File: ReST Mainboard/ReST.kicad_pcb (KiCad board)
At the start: 2 copper layers, 100 x 100 mm, 368 parts, among them P20 CONN_02X04, P21 CONN_02X04, P24 CONN_01X03, P26 CONN_01X03, P28 CONN_01X03, P30 CONN_01X03, P32 CONN_01X03, P34 CONN_01X03, P35 SCREW_01X04, P36 SCREW_01X04, P37 SCREW_01X04, P38 SCREW_01X04, P5 USB_OTG, P9 CONN_01X02, U2 USBLC6-2, U4 LM2574N-ADJ

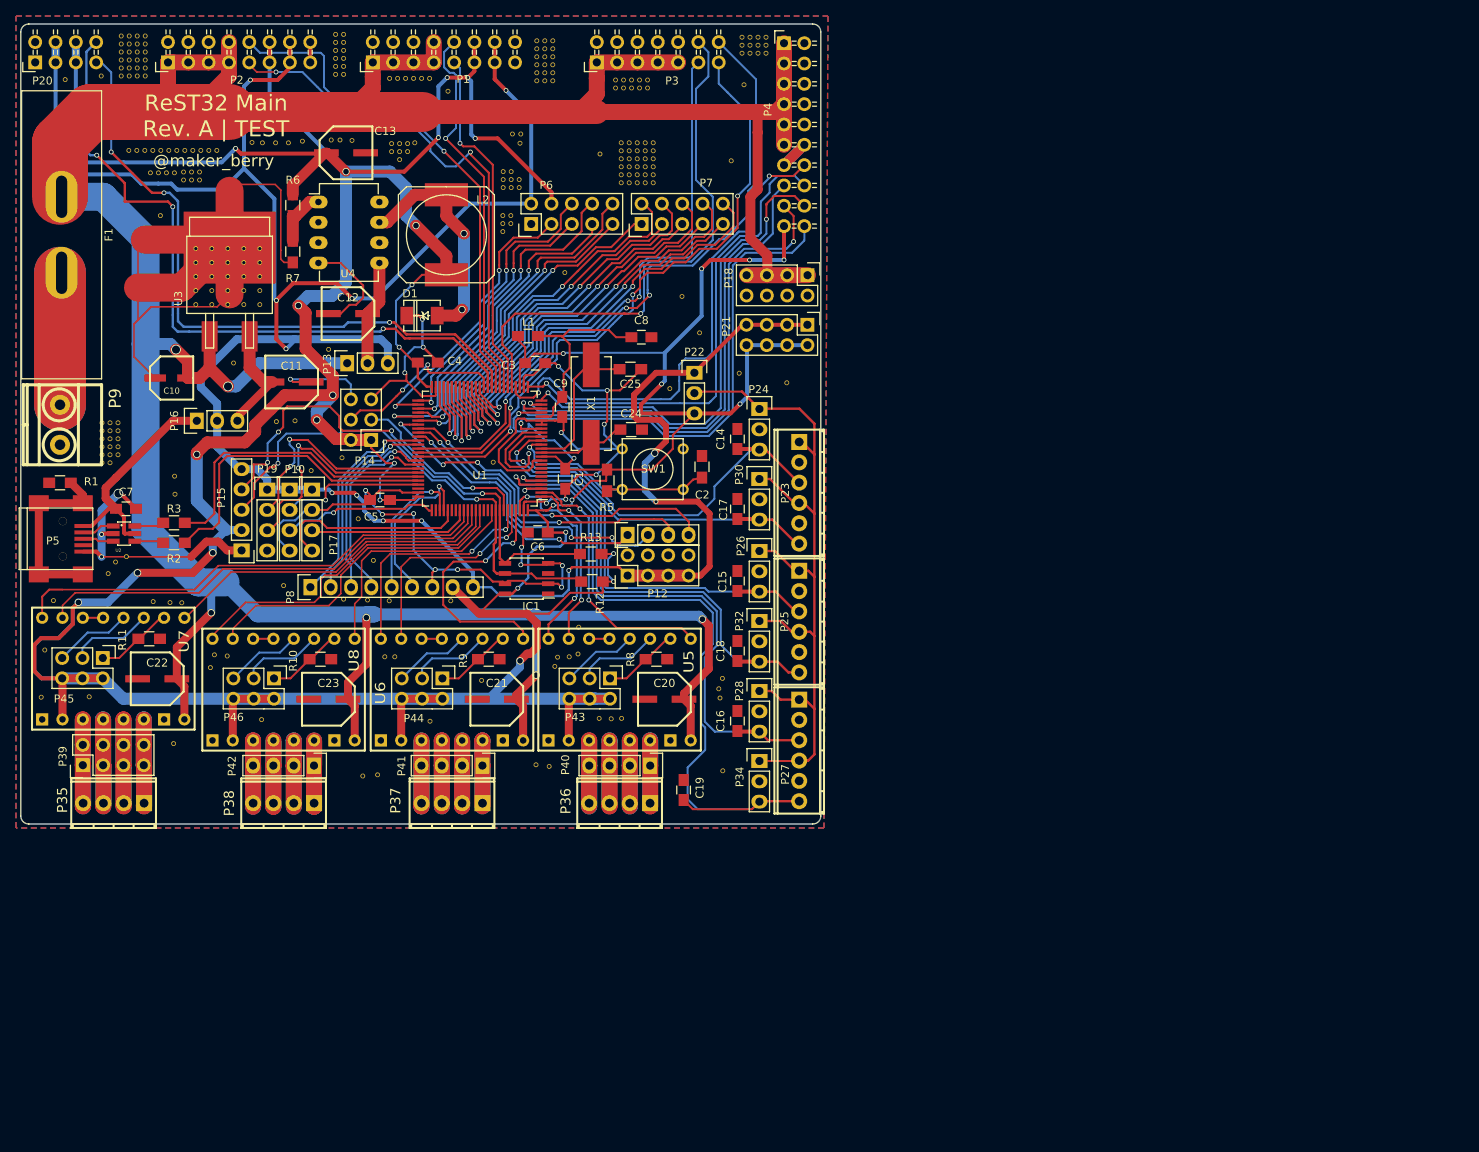
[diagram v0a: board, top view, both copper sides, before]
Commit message: Mainboard structure made and most modules finished
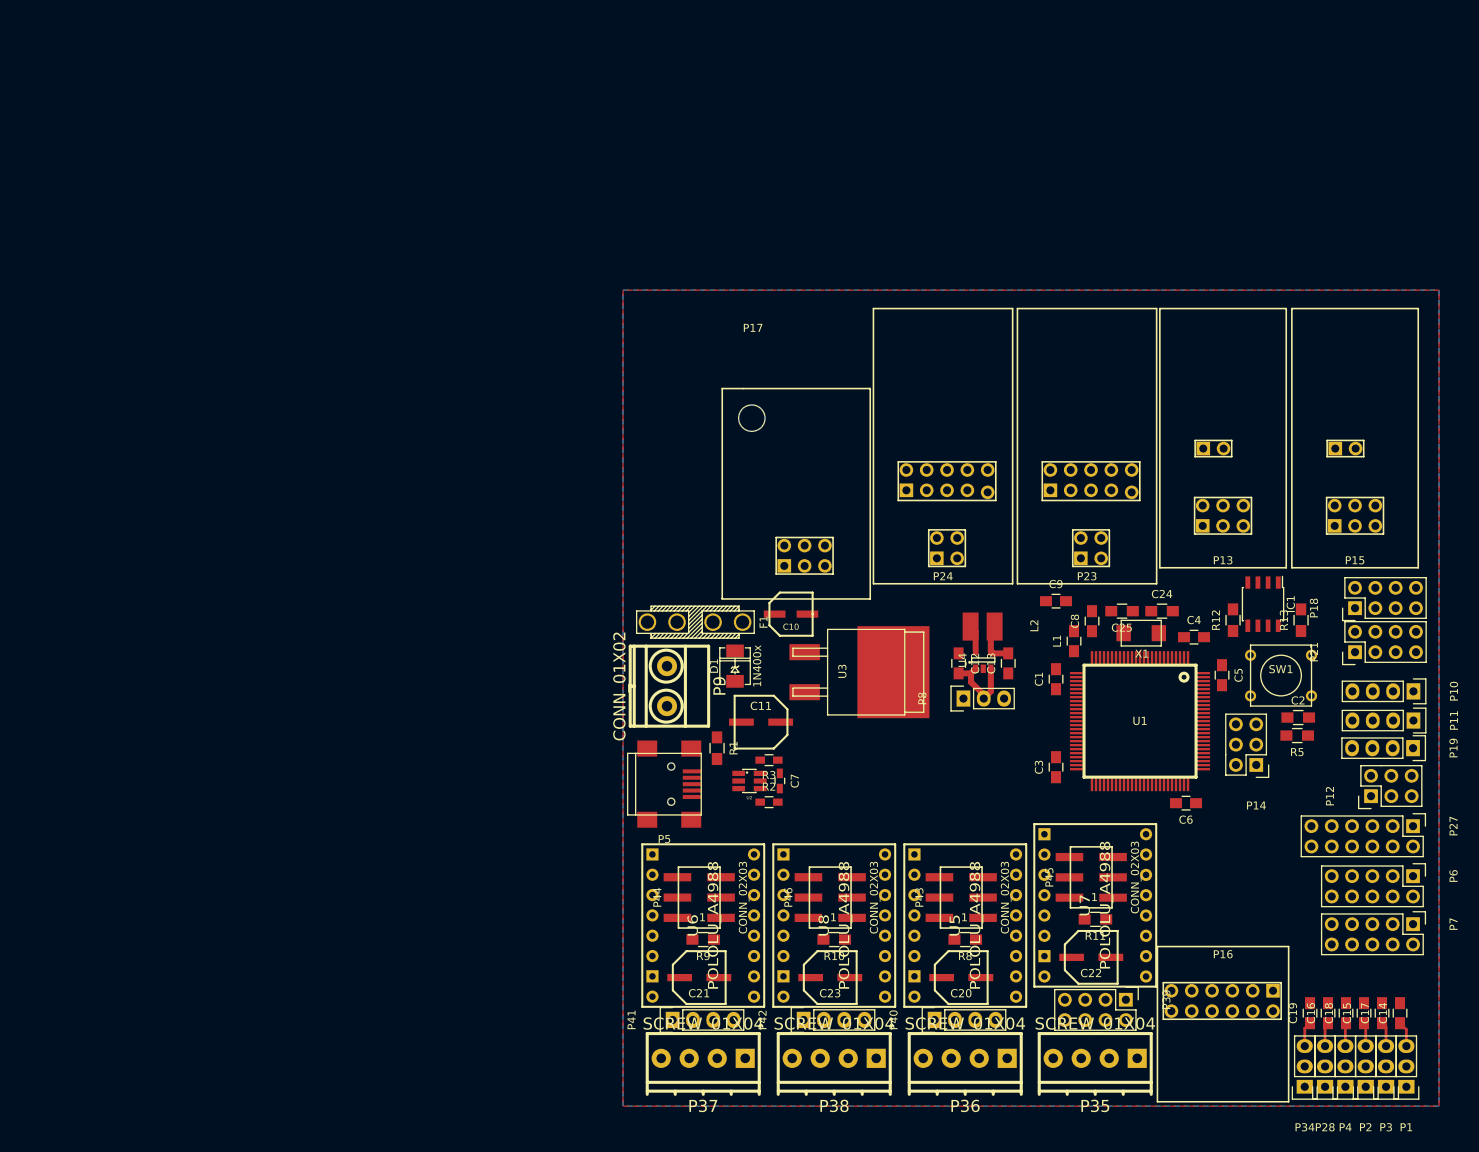
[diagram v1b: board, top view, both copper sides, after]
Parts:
- removed ?: , Pin_Headers:Pin_Header_Straight_1x04
- removed GND (x3), REF**11, REF**111 (x3), REF**11101, REF**1111 (x2), REF**11111 (x2), REF**111111, REF**111112, REF**111113, REF**111114, REF**111115, REF**111116, REF**11112, REF**111121, REF**111122, REF**111123, REF**111124, REF**111125, REF**111126, REF**11113, REF**111131, REF**111132, REF**111133, REF**111134, REF**111135, REF**111136, REF**11114, REF**111141, REF**111142, REF**111143, REF**111144, REF**111145, REF**111146, REF**11115, REF**111151, REF**111152, REF**111153, REF**111154, REF**111155, REF**111156, REF**11116, REF**1112, REF**11121 (x2), REF**11122, REF**11123, REF**11124, REF**11125, REF**11126, REF**1113, REF**1114, REF**1115, REF**1116, REF**112 (x2), REF**1121 (x2), REF**1122, REF**1123, REF**1124, REF**1125, REF**1126, REF**113 (x2), REF**1131 (x2), REF**1132, REF**1133, REF**1134, REF**1135, REF**1136, REF**114 (x2), REF**1141, REF**115 (x2), REF**1151, REF**116 (x2), REF**1161, REF**1171, REF**1181, REF**1191, REF**12, REF**121 (x3), REF**122 (x2), REF**123 (x2), REF**124 (x2), REF**125 (x2), REF**126 (x2), REF**131 (x5), REF**131111 (x6), REF**131112, REF**131113, REF**131114, REF**131115, REF**131121, REF**131122, REF**131123, REF**131124, REF**131125, REF**131131, REF**131132, REF**131133, REF**131134, REF**131135, REF**131141, REF**131142, REF**131143, REF**131144, REF**131145, REF**131151, REF**131152, REF**131153, REF**131154, REF**131155, REF**132 (x2), REF**133 (x2), REF**134 (x2), REF**135 (x2), REF**136, REF**141 (x2), REF**142, REF**143, REF**144, REF**145, REF**146, REF**21, REF**22, REF**31 (x58), REF**311 (x3), REF**3111 (x3), REF**3112 (x2), REF**3113, REF**312 (x3), REF**3121 (x3), REF**3122 (x2), REF**313 (x10), REF**3131 (x2), REF**3132, REF**3141 (x2), REF**3142, REF**3151 (x2), REF**3152, REF**3161, REF**32, REF**321 (x3), REF**322 (x3), REF**323 (x3), REF**331 (x2), REF**332 (x3), REF**333 (x3), REF**341, REF**342, REF**343: VIA-0.6mm, ReST-Library:VIA-0.6mm
- removed GND: , ReST-Library:VIA-0.6mm
- removed P20: CONN_02X04, ReST-Library:Pin_Header_Angled_2x04
- removed P22: , Pin_Headers:Pin_Header_Straight_1x03
- removed P25: , 2:mpt_0,5%2f6-2,54
- removed P26, P30, P32: CONN_01X03, Pin_Headers:Pin_Header_Straight_1x03
- removed R6: 2K7, Resistors_SMD:R_0805_HandSoldering
- removed R7: 1K6, Resistors_SMD:R_0805_HandSoldering
- added P11: CONN_01X04, Pin_Headers:Pin_Header_Straight_1x04, F.Cu at (197.2, 106.8)
- C1, C2, C3, C4, C5, C6, C9: value (none) -> 100nF
- C12: value 22uF -> 10uF; footprint ReST-Library:CP-PANASONIC-SMT_D -> Capacitors_SMD:C_0805_HandSoldering
- C13: value 220uF -> 10uF; footprint ReST-Library:CP-PANASONIC-SMT_D -> Capacitors_SMD:C_0805_HandSoldering
- C14, C15, C16, C17, C18, C19: value (none) -> 10nF
- C24, C25: value (none) -> 30pF
- C7: footprint Capacitors_SMD:C_0805_HandSoldering -> Capacitors_SMD:C_0603_HandSoldering
- C8: value (none) -> 10uF
- D1: value 1N5819 -> 1N400x; footprint ReST-Library:DO-214AC(SMA) -> ReST-Library:DO-214AC.SMA
- F1: footprint ReST-Library:JEF-703C -> ReST-Library:MINI-FUSE
- IC1: value (none) -> AT24C128
- L1: value (none) -> BEAD
- L2: value 330uH -> 2.2uH; footprint Inductors:SELF-WE-PD-XXL -> ReST-Library:CD32
- P1, P2: value (none) -> CONN_01X03; footprint ReST-Library:Pin_Header_Angled_2x08 -> Pin_Headers:Pin_Header_Straight_1x03
- P10, P19, P40, P41, P42: value (none) -> CONN_01X04
- P12: value (none) -> CONN_02X03; footprint Pin_Headers:Pin_Header_Straight_2x04 -> Pin_Headers:Pin_Header_Straight_2x03
- P13: value (none) -> CONN_02X04; footprint Pin_Headers:Pin_Header_Straight_1x03 -> ReST-Library:REST_STEPPER
- P14: value (none) -> CONN_02X03
- P15: value (none) -> CONN_02X04; footprint Pin_Headers:Pin_Header_Straight_1x05 -> ReST-Library:REST_STEPPER
- P16: value (none) -> CONN_02X06; footprint Pin_Headers:Pin_Header_Straight_1x03 -> ReST-Library:REST_ADDITIONAL
- P17: value (none) -> CONN_02X03; footprint Pin_Headers:Pin_Header_Straight_1x04 -> ReST-Library:REST_HEATBED
- P18, P39: value (none) -> CONN_02X04
- P23: value (none) -> CONN_02X07; footprint 2:mpt_0,5%2f6-2,54 -> ReST-Library:REST_HEATER
- P24: value CONN_01X03 -> CONN_02X07; footprint Pin_Headers:Pin_Header_Straight_1x03 -> ReST-Library:REST_HEATER
- P27: value (none) -> CONN_02X06; footprint 2:mpt_0,5%2f6-2,54 -> Pin_Headers:Pin_Header_Straight_2x06
- P3: value (none) -> CONN_01X03; footprint ReST-Library:Pin_Header_Angled_2x07 -> Pin_Headers:Pin_Header_Straight_1x03
- P35, P36, P37, P38: footprint 2:mpt_0,5%2f4-2,54 -> ReST-Library:pt_1,5-4-3,5-h
- P4: value (none) -> CONN_01X03; footprint ReST-Library:Pin_Header_Angled_2x10 -> Pin_Headers:Pin_Header_Straight_1x03
- P43, P44, P45, P46: value (none) -> CONN_02X03; footprint Pin_Headers:Pin_Header_Straight_2x03 -> ReST-Library:bb02-hp06
- P6, P7: value (none) -> CONN_02X05
- P8: value (none) -> CONN_01X03; footprint Pin_Headers:Pin_Header_Straight_1x09 -> Pin_Headers:Pin_Header_Straight_1x03
- P9: footprint 5mm-pitch-terminal:mkds_1,5-2 -> ReST-Library:screw-5-2P
- R10, R11, R8, R9: value (none) -> 100K
- R12, R13: value (none) -> 4K7
- R2, R3: footprint Resistors_SMD:R_0805_HandSoldering -> Resistors_SMD:R_0603_HandSoldering
- R5: value (none) -> 10K
- SW1: value (none) -> SW-SPST-NO
- U1: value (none) -> STM32F103VE; footprint Housings_QFP:TQFP-100_14x14mm_Pitch0.5mm -> ReST-Library:LQFP100-14x14
- U3: value (none) -> L7805ACD2T-TR
- U4: value LM2574N-ADJ -> LM3671MFX-3.3; footprint Housings_DIP:DIP-8_W7.62mm_LongPads -> TO_SOT_Packages_SMD:SOT-23-5
- U5, U6, U7, U8: value (none) -> POLOLU_A4988
- X1: value (none) -> Crystal_Small; footprint Crystals:Crystal_HC49-SD_SMD -> ReST-Library:2P-5032
- moved P2 197.0 mm to (191.3, 152.5), turned to 180 degrees
- moved P1 181.9 mm to (196.4, 152.5), turned to 180 degrees
- moved P3 161.6 mm to (193.8, 152.5), turned to 180 degrees
- moved P16 148.8 mm to (173.4, 144.7), turned to 180 degrees
- moved P4 148.1 mm to (188.7, 152.5), turned to 180 degrees
- moved P19 146.8 mm to (197.2, 110.2), turned to 270 degrees
- moved P10 142.7 mm to (197.2, 103.1), turned to 270 degrees
- moved P15 139.9 mm to (189.9, 71.5), turned to 0 degrees
- moved P6 137.1 mm to (197.2, 126.2), turned to 270 degrees
- moved P39 133.6 mm to (161.3, 141.7), turned to 270 degrees
- moved P7 130.2 mm to (197.2, 132.2), turned to 270 degrees
- moved P35 127.0 mm to (157.5, 149.7)
- moved P45 126.6 mm to (157.0, 126.3), turned to 90 degrees
- moved U7 126.3 mm to (157.5, 129.8), turned to 270 degrees
- moved R11 123.4 mm to (157.5, 131.6), turned to 180 degrees
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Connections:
- net Net-(C2-Pad2) renamed /RESET
- C10 pad 1: GND -> +12V
- C10 pad 2: +12V -> GND
- C11 pad 1: GND -> VEE
- C11 pad 2: VCC/2 -> GND
- C12 pad 1: VAA -> GND
- C12 pad 2: GND -> +5V
- C13 pad 1: +3V3 -> GND
- C13 pad 2: GND -> +3V3
- D1 pad 1: Net-(D1-Pad1) -> +12V
- L2 pad 1: Net-(D1-Pad1) -> Net-(L2-Pad1)
- P1 pad 1: +12V -> +3V3
- P1 pad 3: +12V -> /X-MIN
- P12 pad 1: +5V -> /SERVO1
- P12 pad 2: GND -> /SERVO2
- P12 pad 4: GND -> +5V
- P12 pad 5: +5V -> GND
- P13 pad 1: +12V -> /E1-STEP
- P13 pad 2: VAA -> /E1-EN
- P13 pad 3: +5V -> /E1-DIR
- P15 pad 1: GND -> /E2-STEP
- P15 pad 2: +3V3 -> /E2-EN
- P15 pad 3: /I2C-SCL -> /E2-DIR
- P15 pad 4: /I2C-SDA -> GND
- P15 pad 5: +5V -> +3V3
- P16 pad 1: VCC -> GND
- P16 pad 2: +5V -> GND
- P16 pad 3: VCC/2 -> GND
- P17 pad 2: GND -> +3V3
- P17 pad 3: /UART5-RX -> GND
- P17 pad 4: /UART5-TX -> /PWM-BED
- P2 pad 1: +12V -> +3V3
- P2 pad 3: +12V -> /Y-MIN
- P23 pad 1: /ENDSTOP_VCC -> +3V3
- P23 pad 2: GND -> +5V
- P23 pad 3: /X-MIN -> /T2
- P23 pad 4: /ENDSTOP_VCC -> /PWM-HEAT1
- P23 pad 5: GND -> +12V
- P23 pad 6: /X-MAX -> +12V
- P24 pad 1: /ENDSTOP_VCC -> +3V3
- P24 pad 2: GND -> +5V
- P24 pad 3: /X-MIN -> /T1
- P27 pad 1: /ENDSTOP_VCC -> /EXTRA0
- P27 pad 2: GND -> /EXTRA1
- P27 pad 3: /Z-MIN -> /EXTRA2
- P27 pad 4: /ENDSTOP_VCC -> /EXTRA3
- P27 pad 5: GND -> /EXTRA4
- P27 pad 6: /Z-MAX -> /EXTRA5
- P28 pad 1: /ENDSTOP_VCC -> +3V3
- P3 pad 1: +12V -> +3V3
- P3 pad 3: +12V -> /X-MAX
- P34 pad 1: /ENDSTOP_VCC -> +3V3
- P39 pad 1: Net-(P35-Pad4) -> Net-(P35-Pad1)
- P39 pad 2: Net-(P35-Pad4) -> Net-(P35-Pad1)
- P39 pad 3: Net-(P35-Pad3) -> Net-(P35-Pad2)
- P39 pad 4: Net-(P35-Pad3) -> Net-(P35-Pad2)
- P39 pad 5: Net-(P35-Pad2) -> Net-(P35-Pad3)
- P39 pad 6: Net-(P35-Pad2) -> Net-(P35-Pad3)
- P39 pad 7: Net-(P35-Pad1) -> Net-(P35-Pad4)
- P39 pad 8: Net-(P35-Pad1) -> Net-(P35-Pad4)
- P4 pad 1: +12V -> +3V3
- P4 pad 3: +12V -> /Y-MAX
- P40 pad 1: Net-(P36-Pad1) -> Net-(P36-Pad4)
- P40 pad 2: Net-(P36-Pad2) -> Net-(P36-Pad3)
- P40 pad 3: Net-(P36-Pad3) -> Net-(P36-Pad2)
- P40 pad 4: Net-(P36-Pad4) -> Net-(P36-Pad1)
- P41 pad 1: Net-(P37-Pad1) -> Net-(P37-Pad4)
- P41 pad 2: Net-(P37-Pad2) -> Net-(P37-Pad3)
- P41 pad 3: Net-(P37-Pad3) -> Net-(P37-Pad2)
- P41 pad 4: Net-(P37-Pad4) -> Net-(P37-Pad1)
- P42 pad 1: Net-(P38-Pad1) -> Net-(P38-Pad4)
- P42 pad 2: Net-(P38-Pad2) -> Net-(P38-Pad3)
- P42 pad 3: Net-(P38-Pad3) -> Net-(P38-Pad2)
- P42 pad 4: Net-(P38-Pad4) -> Net-(P38-Pad1)
- P8 pad 1: /EXTRA0 -> VEE
- P8 pad 2: /EXTRA1 -> +5V
- P8 pad 3: /EXTRA2 -> VCC
- U1 pad 59: /SERVO3 -> /EXTRA7
- U1 pad 60: /SERVO4 -> /EXTRA6
- U1 pad 80: /UART5-TX -> /EXTRA8
- U1 pad 81: (no net) -> /EXTRA11
- U1 pad 82: (no net) -> /EXTRA10
- U1 pad 83: /UART5-RX -> /EXTRA9
- U3 pad 3: VCC/2 -> VEE
- U4 pad 1: Net-(R6-Pad2) -> +5V
- U4 pad 2: (no net) -> GND
- U4 pad 3: GND -> +5V
- U4 pad 4: GND -> +3V3
- U4 pad 5: VAA -> Net-(L2-Pad1)
- U5 pad 3: Net-(P36-Pad4) -> Net-(P36-Pad1)
- U5 pad 4: Net-(P36-Pad3) -> Net-(P36-Pad2)
- U5 pad 5: Net-(P36-Pad2) -> Net-(P36-Pad3)
- U5 pad 6: Net-(P36-Pad1) -> Net-(P36-Pad4)
- U6 pad 3: Net-(P37-Pad4) -> Net-(P37-Pad1)
- U6 pad 4: Net-(P37-Pad3) -> Net-(P37-Pad2)
- U6 pad 5: Net-(P37-Pad2) -> Net-(P37-Pad3)
- U6 pad 6: Net-(P37-Pad1) -> Net-(P37-Pad4)
- U7 pad 3: Net-(P35-Pad4) -> Net-(P35-Pad1)
- U7 pad 4: Net-(P35-Pad3) -> Net-(P35-Pad2)
- U7 pad 5: Net-(P35-Pad2) -> Net-(P35-Pad3)
- U7 pad 6: Net-(P35-Pad1) -> Net-(P35-Pad4)
- U8 pad 3: Net-(P38-Pad4) -> Net-(P38-Pad1)
- U8 pad 4: Net-(P38-Pad3) -> Net-(P38-Pad2)
- U8 pad 5: Net-(P38-Pad2) -> Net-(P38-Pad3)
- U8 pad 6: Net-(P38-Pad1) -> Net-(P38-Pad4)
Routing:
- net +3V3: track 649.1 -> 5.56 mm, vias 33 -> 0
- net +12V: track 435.0 -> 0.00 mm, vias 6 -> 0
- net GND: track 332.2 -> 0.00 mm, vias 23 -> 0
- net +5V: track 318.0 -> 10.3 mm, vias 12 -> 0
- net /ENDSTOP_VCC: track 100.1 -> 0.00 mm
- net /PWM-BED: track 88.1 -> 0.00 mm, vias 3 -> 0
- net /Z-MAX: track 88.7 -> 3.14 mm, vias 1 -> 0
- net /PWM-ADD2: track 82.8 -> 0.00 mm, vias 3 -> 0
- net /T0: track 82.6 -> 0.00 mm, vias 3 -> 0
- net /PWM-ADD1: track 79.5 -> 0.00 mm, vias 3 -> 0
- net /PWM-ADD3: track 74.3 -> 0.00 mm, vias 3 -> 0
- net /Z-MIN: track 72.1 -> 3.02 mm, vias 1 -> 0
- net /PWM-ADD0: track 68.9 -> 0.00 mm, vias 1 -> 0
- net /PWM-HEAT0: track 65.6 -> 0.00 mm, vias 2 -> 0
- net /T1: track 64.4 -> 0.00 mm, vias 1 -> 0
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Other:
- board outline removed
- board text removed: "@maker_berry"
- board text removed: "ReST32 Main Rev. A | TEST"
